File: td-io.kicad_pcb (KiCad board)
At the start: 2 copper layers, 66.5 x 54 mm, 18 parts, among them J1 USB_B, J2 I2C, J3 Dips, J4 Test/Service, J5 Power, J6 Controls, Q1 AO4818B, Q2 AO3400A, U1 ISL3175EIBZ-T, U2 Pico

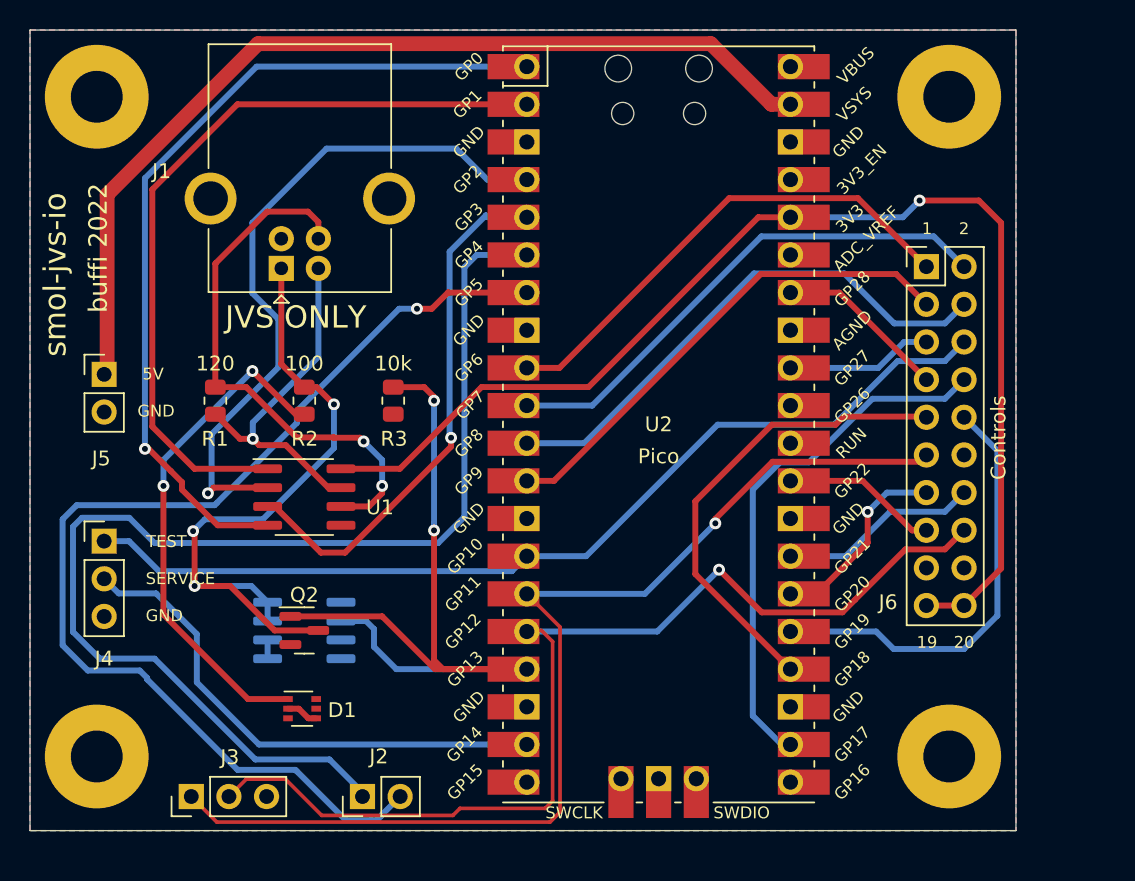
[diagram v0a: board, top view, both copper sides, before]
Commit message: misc stuff
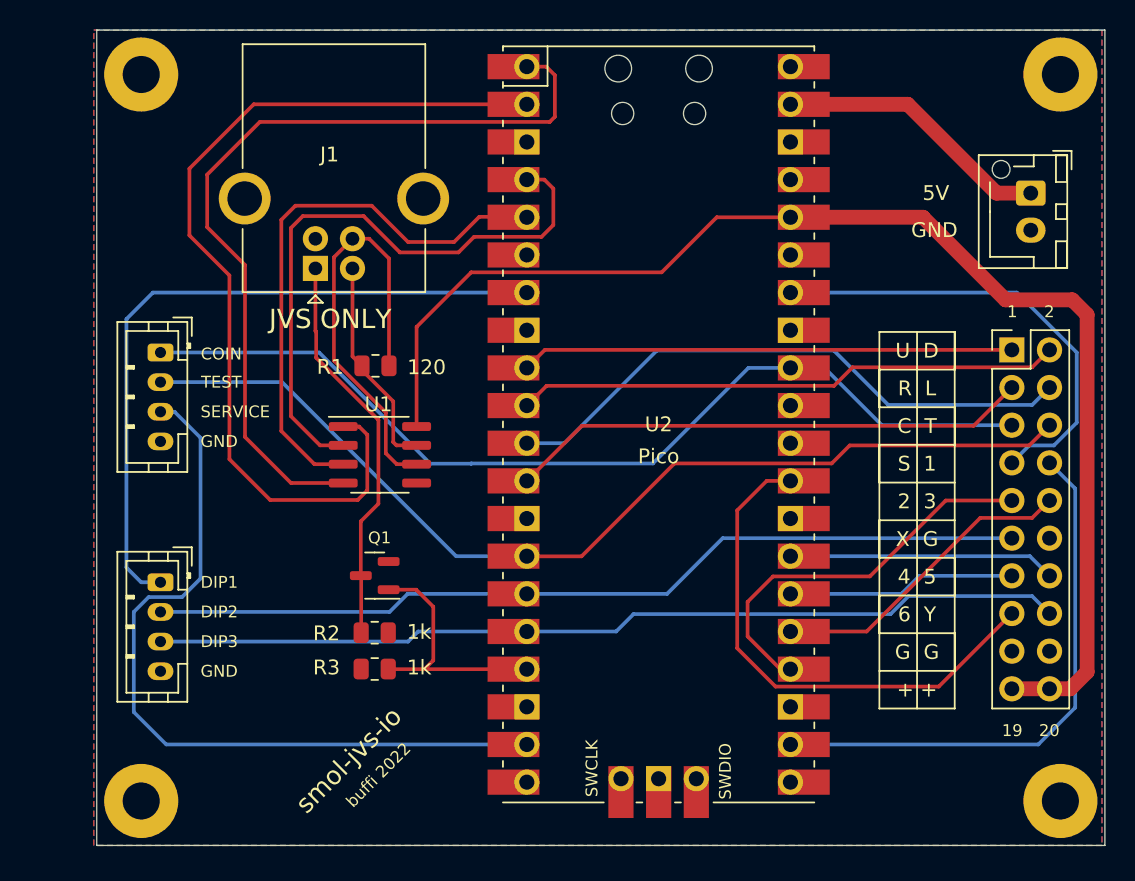
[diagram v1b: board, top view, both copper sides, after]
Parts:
- removed D1: BAV99S, Package_TO_SOT_SMD:SOT-363_SC-70-6
- removed J4: Test/Service, Connector_PinHeader_2.54mm:PinHeader_1x03_P2.54mm_Vertical
- removed the Q1 at (186.0, 84.5)
- H1, H2, H3, H4: footprint MountingHole:MountingHole_3.5mm_Pad -> MountingHole:MountingHole_2.5mm_Pad
- J2: value I2C -> Misc; footprint Connector_PinHeader_2.54mm:PinHeader_1x02_P2.54mm_Vertical -> Connector_JST:JST_PH_B4B-PH-K_1x04_P2.00mm_Vertical
- J3: footprint Connector_PinHeader_2.54mm:PinHeader_1x03_P2.54mm_Vertical -> Connector_JST:JST_PH_B4B-PH-K_1x04_P2.00mm_Vertical
- J5: footprint Connector_PinHeader_2.54mm:PinHeader_1x02_P2.54mm_Vertical -> Connector_JST:JST_XH_B2B-XH-AM_1x02_P2.50mm_Vertical
- R2: value 100 -> 1k
- R3: value 10k -> 1k
- moved J5 63.7 mm to (235.0, 55.0), turned to -90 degrees
- moved J2 32.9 mm to (176.3, 65.8), turned to -90 degrees
- moved R3 18.1 mm to (190.8, 87.1), turned to 180 degrees
- moved R2 16.4 mm to (190.8, 84.7), turned to 0 degrees
- moved J3 14.6 mm to (176.3, 81.2), turned to -90 degrees
- moved R1 11.1 mm to (190.8, 66.7), turned to 180 degrees
- moved H4 8.08 mm to (237.0, 96.0)
- moved J6 8.05 mm to (233.7, 65.6)
- moved H2 7.65 mm to (237.0, 47.0)
- moved Q1 6.02 mm to (190.8, 80.8), turned to 180 degrees
- moved U1 5.84 mm to (191.1, 72.7)
- moved H3 4.24 mm to (175.0, 96.0)
- moved H1 3.35 mm to (175.0, 47.0)
- moved J1 2.30 mm to (186.8, 60.1)
- renumbered Q2 to Q1
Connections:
- H1 pad 1: GND -> unconnected-(H1-Pad1)
- H2 pad 1: GND -> unconnected-(H2-Pad1)
- H3 pad 1: GND -> unconnected-(H3-Pad1)
- H4 pad 1: GND -> unconnected-(H4-Pad1)
- J2 pad 1: Net-(J2-Pad1) -> /b_coin
- J2 pad 2: Net-(J2-Pad2) -> /b_test
- J3 pad 3: GND -> /dip3
- J6 pad 11: /dip1 -> /dip2
- J6 pad 16: /dip2 -> /dip3
- R2 pad 2: Net-(D1-Pad1) -> GND
- U2 pad 15: /dip1 -> /dip2
- U2 pad 16: /dip2 -> /dip3
- U2 pad 6: Net-(J2-Pad1) -> unconnected-(U2-Pad6)
- U2 pad 7: Net-(J2-Pad2) -> /dip1
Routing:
- net Net-(J2-Pad1): track 80.9 -> 0.00 mm
- net Net-(J2-Pad2): track 75.0 -> 0.00 mm, vias 1 -> 0
- net /dip3: track 0.00 -> 61.7 mm
- net /b_coin: track 9.89 -> 64.8 mm
- net +5V: track 64.2 -> 18.7 mm
- net /sense_0v: track 59.3 -> 17.3 mm, vias 2 -> 0
- net Net-(D1-Pad1): track 34.4 -> 0.00 mm, vias 2 -> 0
- net /dip1: track 72.5 -> 47.2 mm, vias 1 -> 0
- net /b_6: track 10.6 -> 35.4 mm
- net /b_start: track 11.6 -> 31.2 mm
- net /jvs_sense: track 45.9 -> 26.8 mm, vias 3 -> 0
- net /b_service: track 35.0 -> 52.5 mm
- net /dip2: track 71.3 -> 59.5 mm, vias 1 -> 0
- net Net-(J1-Pad2): track 23.9 -> 14.5 mm, vias 1 -> 0
- net /jvs_rx: track 52.6 -> 61.6 mm
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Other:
- board size 66.5 x 54 mm -> 68 x 55 mm
- board text added: "+ +"
- board text added: "2 3"
- board text added: "4 5"
- board text added: "6 Y"
- board text added: "C T"
- board text added: "COIN"
- board text added: "DIP1"
- board text added: "DIP2"
- board text added: "DIP3"
- board text added: "G G"
- board text added: "R L"
- board text added: "S 1"
- board text added: "U D"
- board text added: "X G"
- board text removed: "Alternative footprint"
